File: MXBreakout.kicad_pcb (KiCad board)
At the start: 2 copper layers, 27.9 x 19 mm, 12 parts, among them U1 Wii-MX, X1 32.768kHz

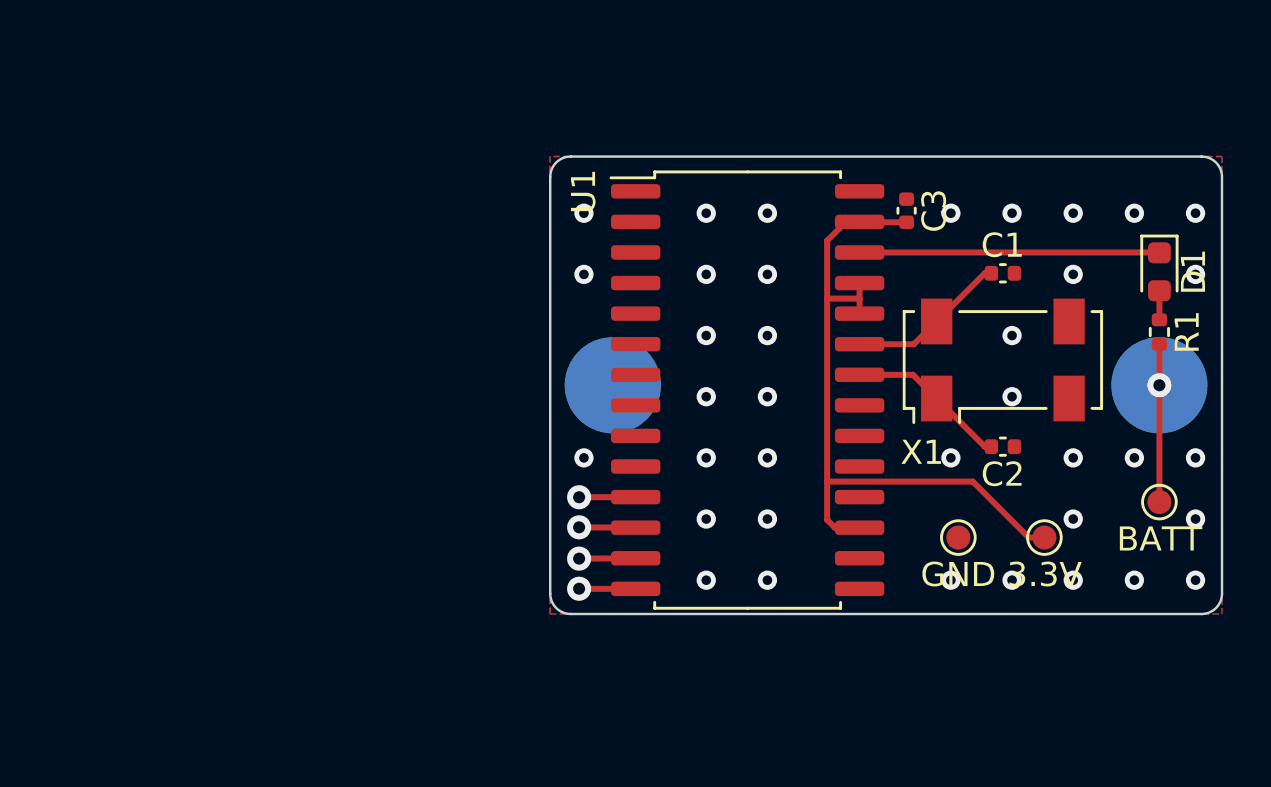
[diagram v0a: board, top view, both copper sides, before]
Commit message: nearing completion
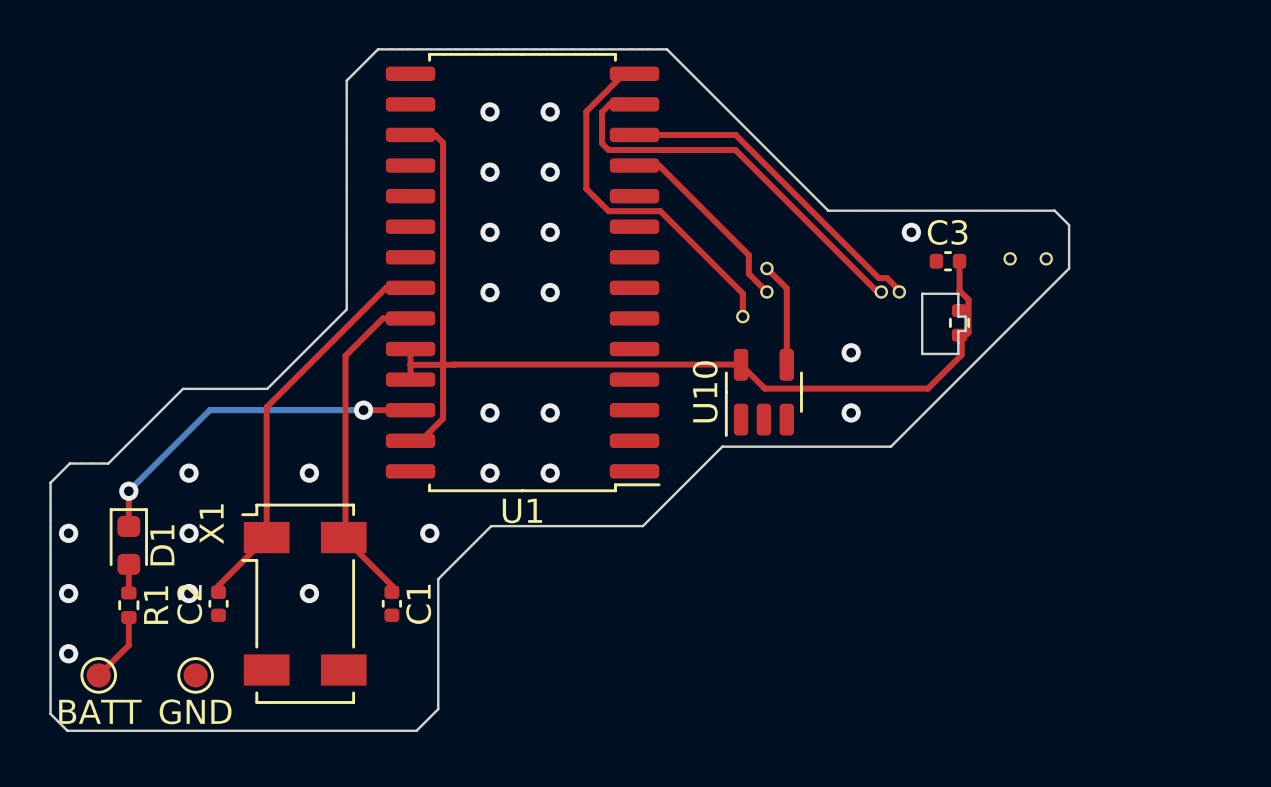
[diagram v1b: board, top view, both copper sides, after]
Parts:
- removed TP1: BATT, TestPoint:TestPoint_Pad_D4.0mm
- removed TP9: 3.3V, TestPoint:TestPoint_Pad_D1.0mm
- added TP10: TestPoint_2Pole, Resistor_SMD:R_0402_1005Metric, F.Cu at (132.0, 86.3)
- added TP11: U10, Wii:TestPoint_THTPad_D0.5mm_Drill0.35mm, F.Cu at (124.0, 84.0)
- added TP3: GND, Wii:TestPoint_THTPad_D0.5mm_Drill0.35mm, F.Cu at (135.6, 83.6)
- added TP4: TestPoint, Wii:TestPoint_THTPad_D0.5mm_Drill0.35mm, F.Cu at (124.0, 85.0)
- added TP5: TestPoint, Wii:TestPoint_THTPad_D0.5mm_Drill0.35mm, F.Cu at (129.5, 85.0)
- added TP6: TestPoint, Wii:TestPoint_THTPad_D0.5mm_Drill0.35mm, F.Cu at (128.8, 85.0)
- added TP7: TestPoint, Wii:TestPoint_THTPad_D0.5mm_Drill0.35mm, F.Cu at (123.0, 86.0)
- added U10: ~, Package_TO_SOT_SMD:SOT-23-5, F.Cu at (123.9, 89.1)
- TP2: footprint TestPoint:TestPoint_Pad_D4.0mm -> TestPoint:TestPoint_Pad_D1.0mm; moved to F.Cu
- TP3: footprint TestPoint:TestPoint_Pad_D1.0mm -> Wii:TestPoint_THTPad_D0.5mm_Drill0.35mm
- moved TP8 44.6 mm to (96.2, 100.9)
- moved D1 44.3 mm to (97.5, 95.5)
- moved R1 44.3 mm to (97.5, 98.0)
- moved C2 33.2 mm to (101.2, 97.9), turned to 90 degrees
- moved X1 30.7 mm to (104.8, 97.9), turned to 0 degrees
- moved C1 28.8 mm to (108.4, 97.9), turned to 90 degrees
- moved TP2 21.1 mm to (100.3, 100.9), turned to 0 degrees
- moved TP3 11.8 mm to (134.1, 83.6)
- moved U1 10.5 mm to (113.8, 84.2), turned to 180 degrees
- moved C3 2.71 mm to (131.5, 83.7), turned to 0 degrees
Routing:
- net +3.3V: track 30.0 -> 44.9 mm
- net /DATA2: track 2.37 -> 16.9 mm, vias 1 -> 0
- net /DATA3: track 2.33 -> 15.1 mm, vias 1 -> 0
- net /DATA1: track 2.37 -> 13.7 mm, vias 1 -> 0
- net Net-(U1-X_2): track 6.71 -> 16.5 mm
- net Net-(U1-X_1): track 6.69 -> 14.0 mm
- net /DATA0: track 2.36 -> 8.13 mm, vias 1 -> 0
- net Net-(U10-RST): track 0.00 -> 4.34 mm
- net Net-(R1-Pad2): track 6.55 -> 2.92 mm, vias 1 -> 0
- net Net-(D1-K): track 12.5 -> 14.6 mm, vias 0 -> 2
- net GND: vias 37 -> 24
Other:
- board size 27.9 x 19 mm -> 42.3 x 28.3 mm
